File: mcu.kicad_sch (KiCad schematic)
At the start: 34 parts, among them J1 U.FL-R-SMT-1(10), U1 SF32LB525UC6, U2 MKDV1GCL-ABA, Y1 48MHz, Y2 32.768khz

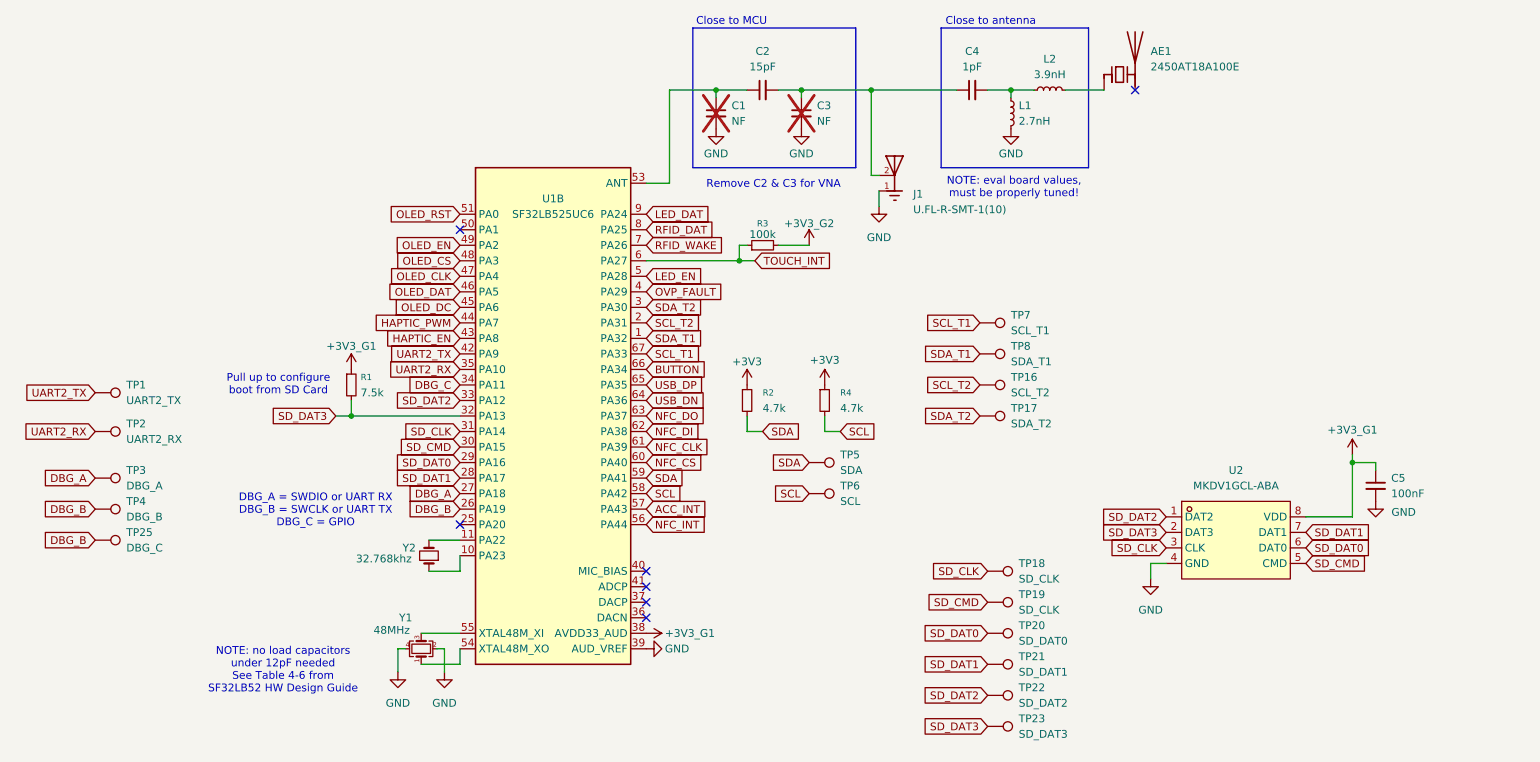
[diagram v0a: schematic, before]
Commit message: huge progress on bentoboard, schematic fixes
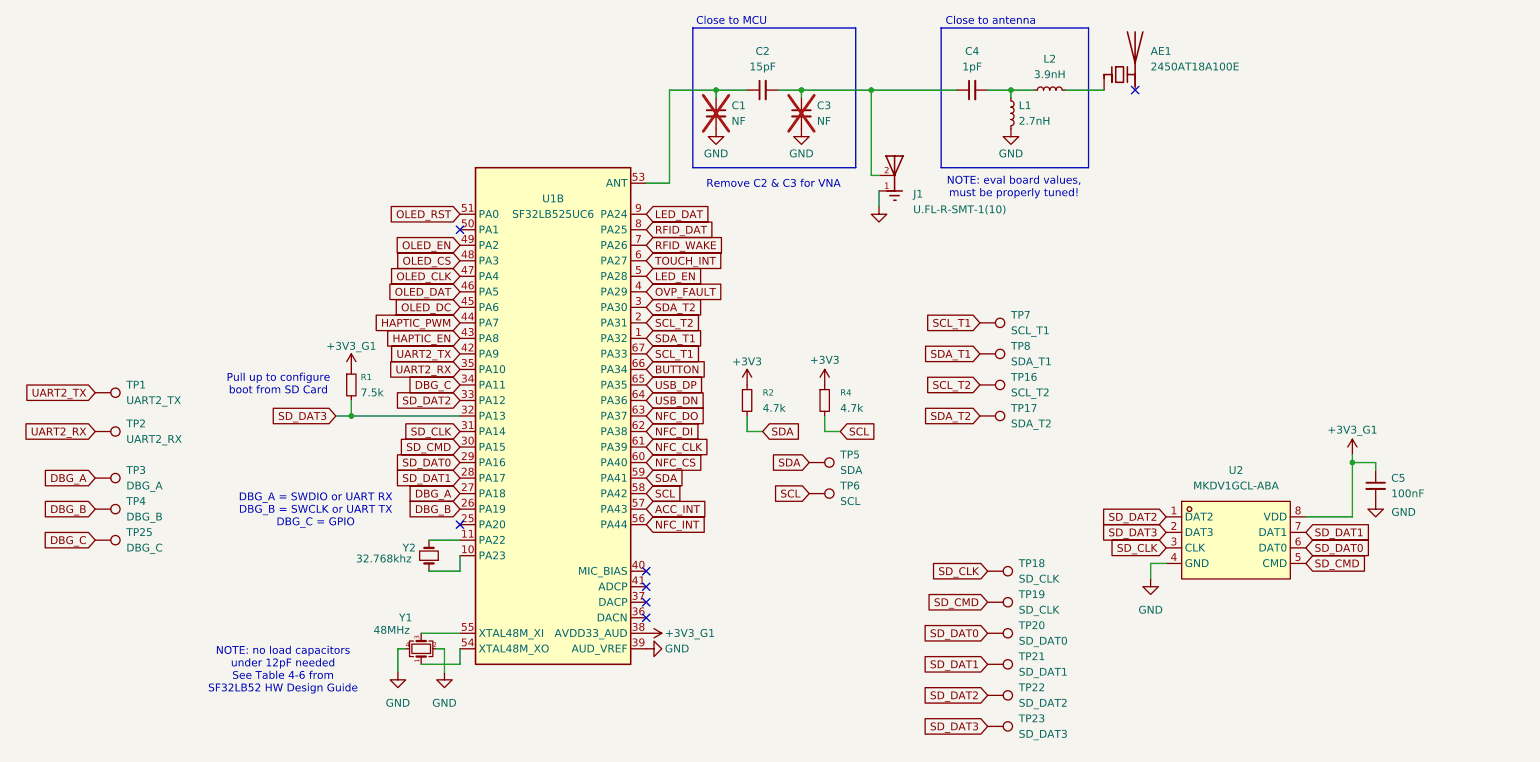
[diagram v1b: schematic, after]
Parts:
- removed R3: 100k, Resistor_SMD:R_0402_1005Metric, symbol Device:R_Small
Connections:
- net DBG_B: no longer TP25.1
- net DBG_C: now also TP25.1
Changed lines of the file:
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@@
 	)
 	(junction
-		(at 152.4 78.74)
-		(diameter 0)
-		(color 0 0 0 0)
-	)
-	(junction
 		(at 148.59 50.8)
 		(diameter 0)
@@
 	(wire
 		(pts
-			(xy 152.4 76.2) (xy 152.4 78.74)
-		)
-		(stroke
-			(width 0)
-			(type default)
-		)
-	)
-	(wire
-		(pts
 			(xy 166.37 106.68) (xy 168.91 106.68)
 		)
@@
 	(wire
 		(pts
-			(xy 158.75 76.2) (xy 163.83 76.2)
-		)
-		(stroke
-			(width 0)
-			(type default)
-		)
-	)
-	(wire
-		(pts
 			(xy 148.59 50.8) (xy 148.59 52.07)
 		)
@@
 	(wire
 		(pts
-			(xy 152.4 78.74) (xy 154.94 78.74)
-		)
-		(stroke
-			(width 0)
-			(type default)
-		)
-	)
-	(wire
-		(pts
 			(xy 100.33 139.7) (xy 106.68 139.7)
 		)
@@
 	(wire
 		(pts
-			(xy 153.67 76.2) (xy 152.4 76.2)
-		)
-		(stroke
-			(width 0)
-			(type default)
-		)
-	)
-	(wire
-		(pts
 			(xy 256.54 111.76) (xy 252.73 111.76)
 		)
@@
 	(wire
 		(pts
-			(xy 137.16 78.74) (xy 152.4 78.74)
-		)
-		(stroke
-			(width 0)
-			(type default)
-		)
-	)
-	(wire
-		(pts
 			(xy 101.6 124.46) (xy 106.68 124.46)
 		)
@@
 		)
 	)
+	(global_label "TOUCH_INT"
+		(shape input)
+		(at 137.16 78.74 0)
+		(fields_autoplaced yes)
+		(effects
+			(font
+				(size 1.27 1.27)
+			)
+			(justify left)
+		)
+		(property "Intersheetrefs" "${INTERSHEET_REFS}"
+			(at 150.2448 78.74 0)
+			(effects
+				(font
+					(size 1.27 1.27)
+				)
+				(justify left)
+				(hide yes)
+			)
+		)
+	)
 	(global_label "OLED_DAT"
 		(shape input)
@@
 		)
 	)
-	(global_label "DBG_B"
+	(global_label "DBG_C"
 		(shape input)
 		(at 46.99 124.46 180)
@@
 		)
 	)
-	(global_label "TOUCH_INT"
-		(shape input)
-		(at 154.94 78.74 0)
-		(fields_autoplaced yes)
-		(effects
-			(font
-				(size 1.27 1.27)
-			)
-			(justify left)
-		)
-		(property "Intersheetrefs" "${INTERSHEET_REFS}"
-			(at 168.0248 78.74 0)
-			(effects
-				(font
-					(size 1.27 1.27)
-				)
-				(justify left)
-				(hide yes)
-			)
-		)
-	)
 	(global_label "SDA"
 		(shape input)
@@
 	)
 	(symbol
-		(lib_id "custom_syms:+3V3_G2")
-		(at 163.83 76.2 0)
-		(unit 1)
-		(exclude_from_sim no)
-		(in_bom yes)
-		(on_board yes)
-		(dnp no)
-		(property "Reference" "#PWR09"
-			(at 163.83 80.01 0)
-			(effects
-				(font
-					(size 1.27 1.27)
-				)
-				(hide yes)
-			)
-		)
-		(property "Value" "+3V3_G2"
-			(at 163.83 72.644 0)
-			(effects
-				(font
-					(size 1.27 1.27)
-				)
-			)
-		)
-		(property "Footprint" ""
-			(at 163.83 76.2 0)
-			(effects
-				(font
-					(size 1.27 1.27)
-				)
-				(hide yes)
-			)
-		)
-		(property "Datasheet" ""
-			(at 163.83 76.2 0)
-			(effects
-				(font
-					(size 1.27 1.27)
-				)
-				(hide yes)
-			)
-		)
-		(property "Description" "Power symbol creates a global label with name \"+3V3_G2\""
-			(at 163.83 76.2 0)
-			(effects
-				(font
-					(size 1.27 1.27)
-				)
-				(hide yes)
-			)
-		)
-		(pin "1"
-		)
-		(instances
-			(project ""
-				(path "/c6cb5a1d-9f97-4766-8582-a9e93ed049e4/c4c0fb03-7c4b-4d55-99ac-6edbef8e602c"
-					(reference "#PWR09")
-					(unit 1)
-				)
-			)
-		)
-	)
-	(symbol
 		(lib_id "Connector:TestPoint")
 		(at 46.99 100.33 270)
@@
 					(size 1.27 1.27)
 				)
+				(hide yes)
 			)
 		)
@@
 					(unit 1)
 				)
-			)
-		)
-	)
-	(symbol
-		(lib_id "Device:R_Small")
-		(at 156.21 76.2 90)
-		(unit 1)
-		(exclude_from_sim no)
-		(in_bom yes)
-		(on_board yes)
-		(dnp no)
-		(property "Reference" "R3"
-			(at 156.21 72.644 90)
-			(effects
-				(font
-					(size 1.016 1.016)
-				)
-			)
-		)
-		(property "Value" "100k"
-			(at 156.21 74.422 90)
-			(effects
-				(font
-					(size 1.27 1.27)
-				)
-			)
-		)
-		(property "Footprint" "Resistor_SMD:R_0402_1005Metric"
-			(at 156.21 76.2 0)
-			(effects
-				(font
-					(size 1.27 1.27)
-				)
-				(hide yes)
-			)
-		)
-		(property "Datasheet" "~"
-			(at 156.21 76.2 0)
-			(effects
-				(font
-					(size 1.27 1.27)
-				)
-				(hide yes)
-			)
-		)
-		(property "Description" "Resistor, small symbol"
-			(at 156.21 76.2 0)
-			(effects
-				(font
-					(size 1.27 1.27)
-				)
-				(hide yes)
-			)
-		)
-		(property "LCSC Part" "C25741"
-			(at 156.21 76.2 90)
-			(effects
-				(font
-					(size 1.27 1.27)
-				)
-				(hide yes)
-			)
-		)
-		(property "CREATOR" ""
-			(at 156.21 76.2 90)
-			(effects
-				(font
-					(size 1.27 1.27)
-				)
-				(hide yes)
-			)
-		)
-		(property "MAXIMUM_PACKAGE_HEIGHT" ""
-			(at 156.21 76.2 90)
-			(effects
-				(font
-					(size 1.27 1.27)
-				)
-				(hide yes)
-			)
-		)
-		(property "PARTREV" ""
-			(at 156.21 76.2 90)
-			(effects
-				(font
-					(size 1.27 1.27)
-				)
-				(hide yes)
-			)
-		)
-		(property "VERIFIER" ""
-			(at 156.21 76.2 90)
-			(effects
-				(font
-					(size 1.27 1.27)
-				)
-				(hide yes)
-			)
-		)
-		(pin "2"
-		)
-		(pin "1"
-		)
-		(instances
-			(project ""
-				(path "/c6cb5a1d-9f97-4766-8582-a9e93ed049e4/c4c0fb03-7c4b-4d55-99ac-6edbef8e602c"
-					(reference "R3")
-					(unit 1)
-				)

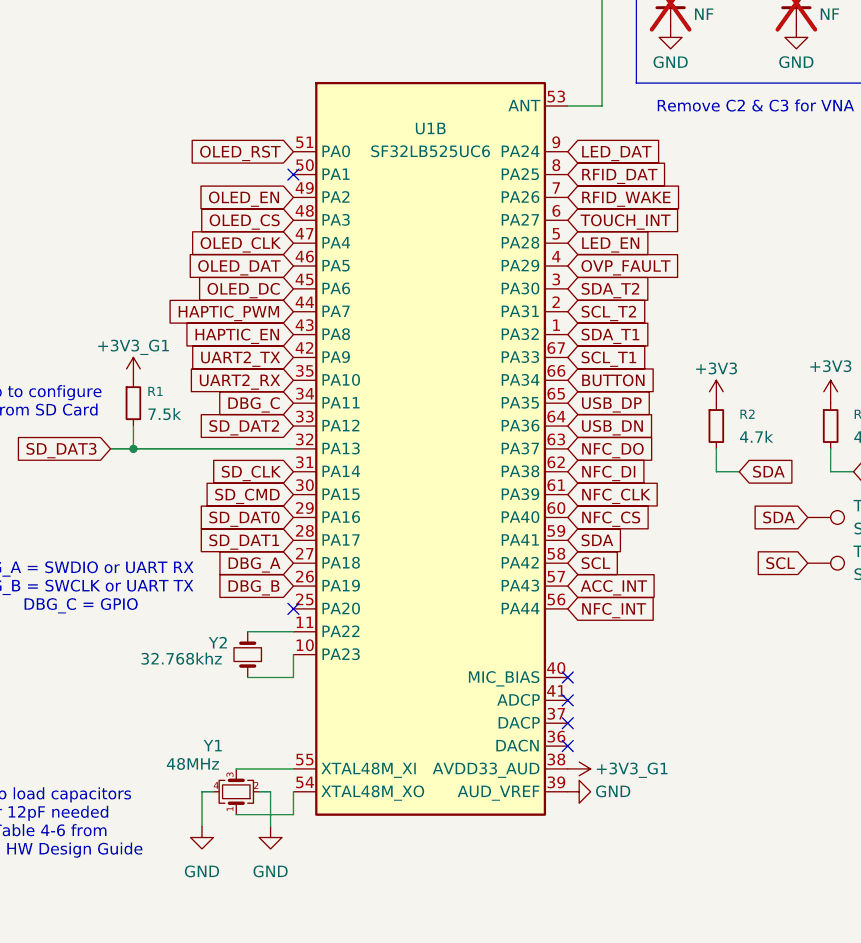
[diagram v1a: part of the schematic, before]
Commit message: rev1 done hopefully
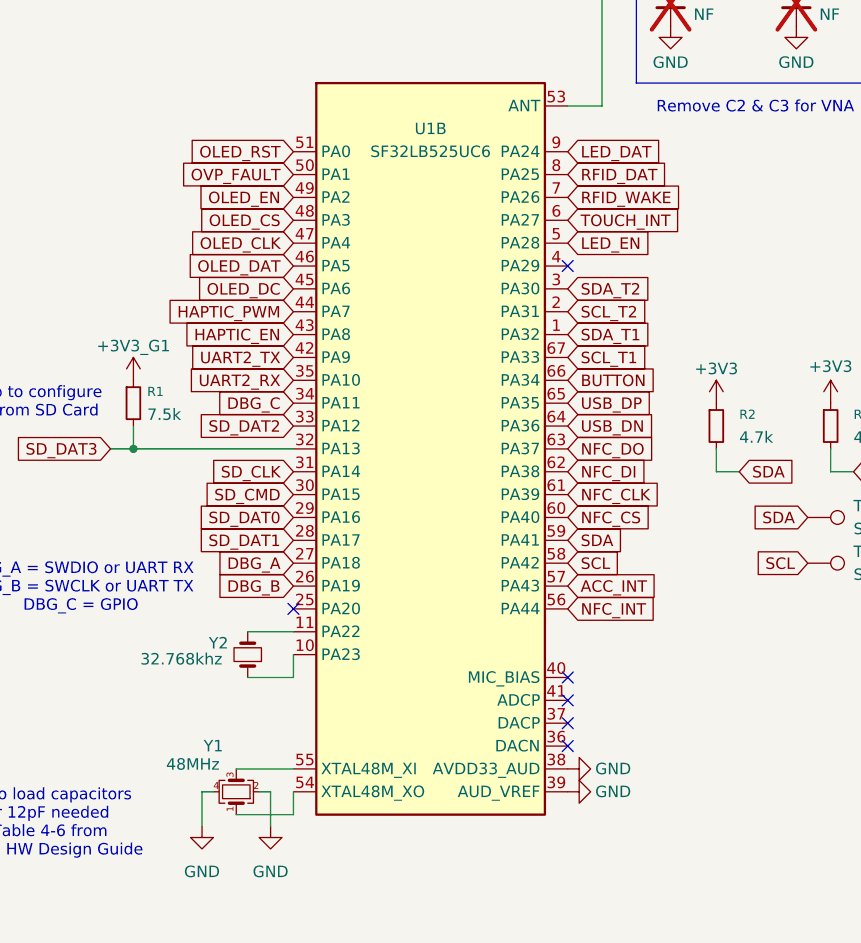
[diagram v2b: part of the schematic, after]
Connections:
- net +3V3_G1: no longer U1.38 (AVDD33_AUD)
- net GND: now also U1.38 (AVDD33_AUD)
- net OVP_FAULT: now also U1.50 (PA1); no longer U1.4 (PA29)
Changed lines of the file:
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@@
 	)
 	(no_connect
-		(at 137.16 129.54)
+		(at 137.16 83.82)
 	)
 	(no_connect
-		(at 106.68 73.66)
+		(at 137.16 129.54)
 	)
 	(wire
@@
 	(global_label "OVP_FAULT"
 		(shape input)
-		(at 137.16 83.82 0)
+		(at 106.68 73.66 180)
 		(fields_autoplaced yes)
 		(effects
@@
 				(size 1.27 1.27)
 			)
-			(justify left)
+			(justify right)
 		)
 		(property "Intersheetrefs" "${INTERSHEET_REFS}"
-			(at 150.3053 83.82 0)
+			(at 93.5347 73.66 0)
 			(effects
 				(font
 					(size 1.27 1.27)
 				)
-				(justify left)
+				(justify right)
 				(hide yes)
 			)
@@
 	)
 	(symbol
+		(lib_id "power:GND")
+		(at 137.16 139.7 90)
+		(unit 1)
+		(exclude_from_sim no)
+		(in_bom yes)
+		(on_board yes)
+		(dnp no)
+		(property "Reference" "#PWR04"
+			(at 143.51 139.7 0)
+			(effects
+				(font
+					(size 1.27 1.27)
+				)
+				(hide yes)
+			)
+		)
+		(property "Value" "GND"
+			(at 140.208 139.7 90)
+			(effects
+				(font
+					(size 1.27 1.27)
+				)
+				(justify right)
+			)
+		)
+		(property "Footprint" ""
+			(at 137.16 139.7 0)
+			(effects
+				(font
+					(size 1.27 1.27)
+				)
+				(hide yes)
+			)
+		)
+		(property "Datasheet" ""
+			(at 137.16 139.7 0)
+			(effects
+				(font
+					(size 1.27 1.27)
+				)
+				(hide yes)
+			)
+		)
+		(property "Description" "Power symbol creates a global label with name \"GND\" , ground"
+			(at 137.16 139.7 0)
+			(effects
+				(font
+					(size 1.27 1.27)
+				)
+				(hide yes)
+			)
+		)
+		(pin "1"
+		)
+		(instances
+			(project ""
+				(path "/c6cb5a1d-9f97-4766-8582-a9e93ed049e4/c4c0fb03-7c4b-4d55-99ac-6edbef8e602c"
+					(reference "#PWR04")
+					(unit 1)
+				)
+			)
+		)
+	)
+	(symbol
 		(lib_id "PCM_MCU_SiFli:SF32LB52xUx")
 		(at 121.92 104.14 0)
@@
 					(unit 1)
 				)
-			)
-		)
-	)
-	(symbol
-		(lib_id "custom_syms:+3V3_G1")
-		(at 137.16 139.7 270)
-		(unit 1)
-		(exclude_from_sim no)
-		(in_bom yes)
-		(on_board yes)
-		(dnp no)
-		(property "Reference" "#PWR04"
-			(at 133.35 139.7 0)
-			(effects
-				(font
-					(size 1.27 1.27)
-				)
-				(hide yes)
-			)
-		)
-		(property "Value" "+3V3_G1"
-			(at 140.208 139.7 90)
-			(effects
-				(font
-					(size 1.27 1.27)
-				)
-				(justify left)
-			)
-		)
-		(property "Footprint" ""
-			(at 137.16 139.7 0)
-			(effects
-				(font
-					(size 1.27 1.27)
-				)
-				(hide yes)
-			)
-		)
-		(property "Datasheet" ""
-			(at 137.16 139.7 0)
-			(effects
-				(font
-					(size 1.27 1.27)
-				)
-				(hide yes)
-			)
-		)
-		(property "Description" "Power symbol creates a global label with name \"+3V3_G1\""
-			(at 137.16 139.7 0)
-			(effects
-				(font
-					(size 1.27 1.27)
-				)
-				(hide yes)
-			)
-		)
-		(pin "1"
-		)
-		(instances
-			(project ""
-				(path "/c6cb5a1d-9f97-4766-8582-a9e93ed049e4/c4c0fb03-7c4b-4d55-99ac-6edbef8e602c"
-					(reference "#PWR04")
-					(unit 1)
-				)

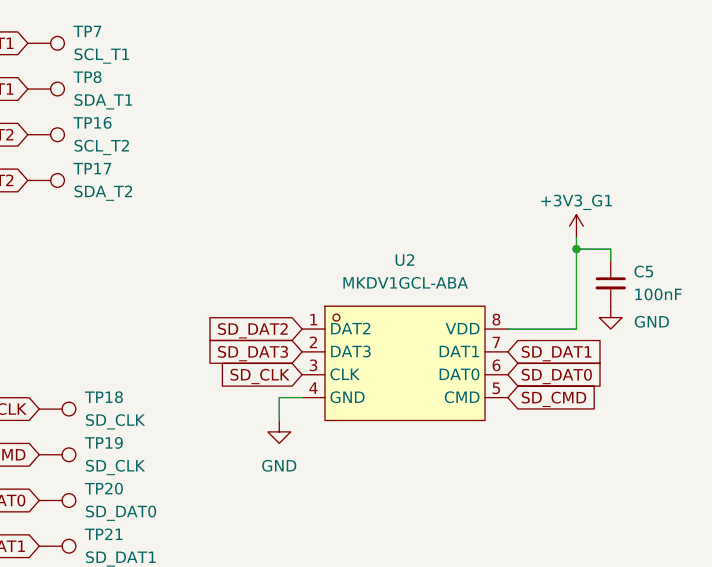
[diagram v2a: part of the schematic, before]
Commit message: fixups before manufacturing pt1
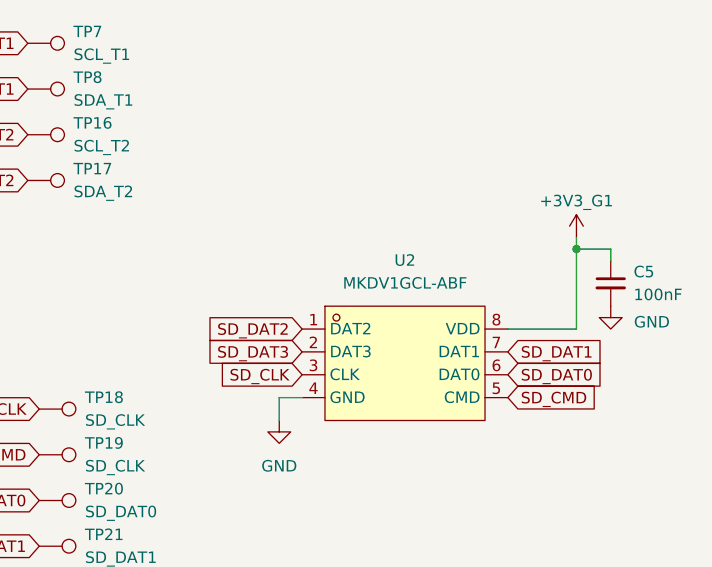
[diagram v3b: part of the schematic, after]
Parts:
- U2: value MKDV1GCL-ABA -> MKDV1GCL-ABF; LCSC Part C6152616 -> C51966230
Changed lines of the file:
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@@
 			)
 		)
-		(property "Value" "MKDV1GCL-ABA"
+		(property "Value" "MKDV1GCL-ABF"
 			(at 233.68 115.57 0)
 			(effects
@@
 			)
 		)
-		(property "LCSC Part" "C6152616"
+		(property "LCSC Part" "C51966230"
 			(at 233.68 138.43 0)
 			(effects
